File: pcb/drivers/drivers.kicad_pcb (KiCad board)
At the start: 2 copper layers, 51.4 x 53.3 mm, 20 parts, among them J1 Conn_01x04_Male, J2 Conn_01x04_Male, J3 Conn_01x04_Male, J4 Conn_01x04_Male, J5 Conn_01x04_Male, J6 Conn_01x02_Male, J7 Conn_01x12_Female, J8 Conn_01x12_Female, Q1 IRLML6402, Q2 IRLML6402, Q3 IRLML6402, Q4 IRLML6402, Q5 IRLML6402

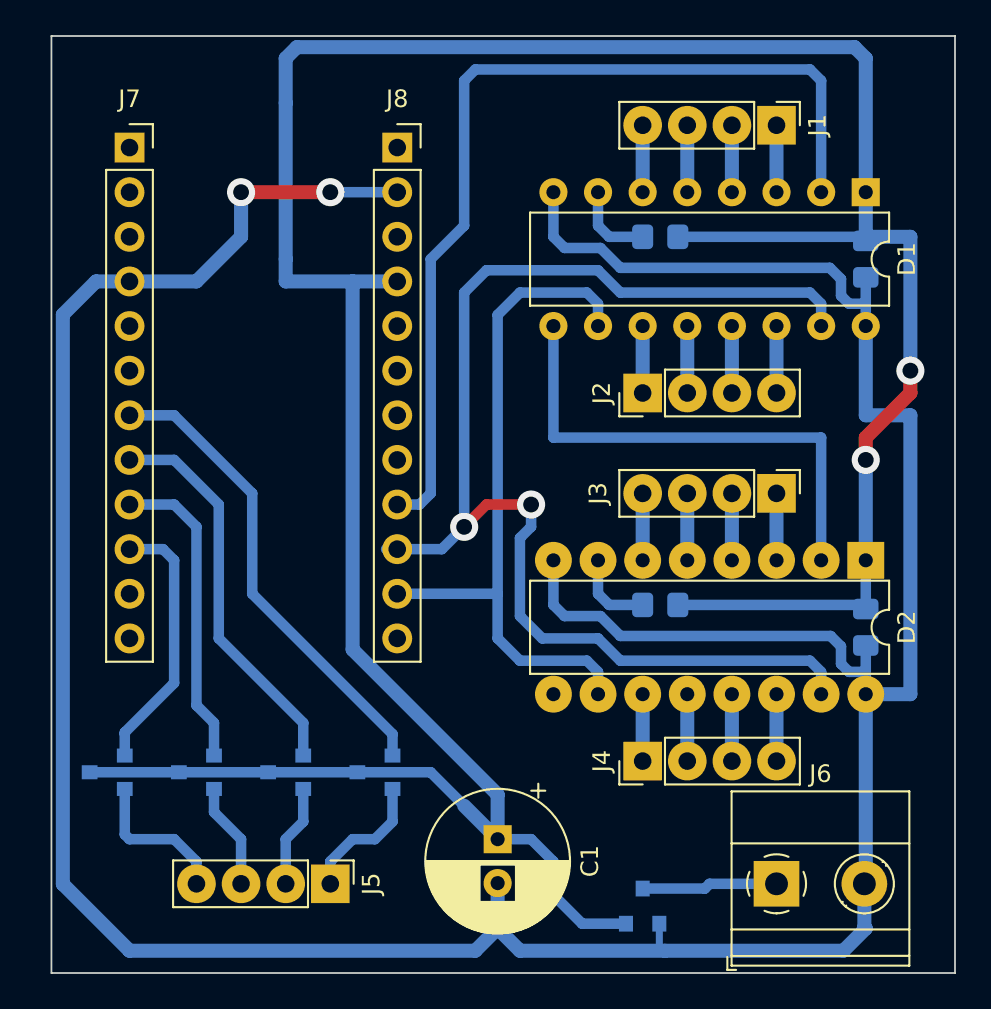
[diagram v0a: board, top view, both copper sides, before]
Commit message: Polishing
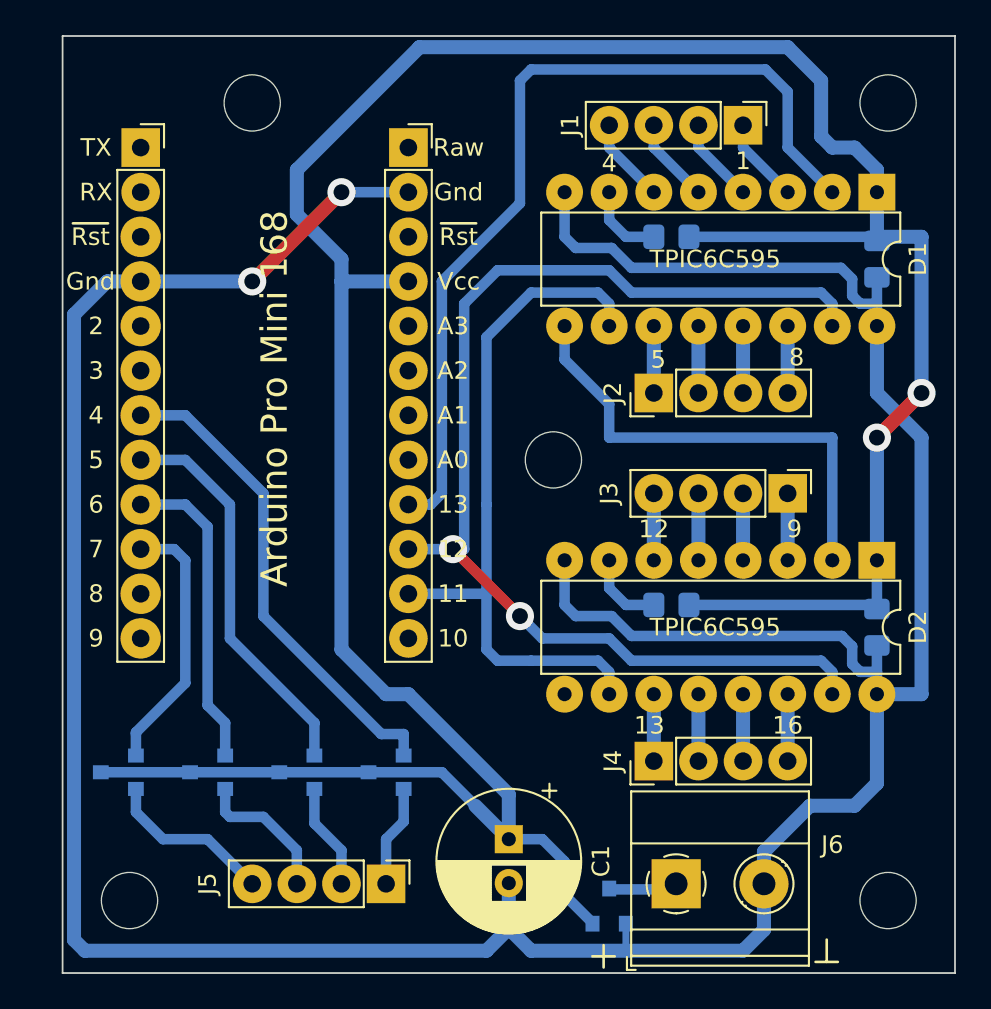
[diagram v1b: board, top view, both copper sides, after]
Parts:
- added H1: MountingHole, MountingHole:MountingHole_3.2mm_M3, F.Cu at (71.8, 31.8)
- added H2: MountingHole, MountingHole:MountingHole_3.2mm_M3, F.Cu at (88.9, 52.1)
- added H3: MountingHole, MountingHole:MountingHole_3.2mm_M3, F.Cu at (108.0, 31.8)
- added H4: MountingHole, MountingHole:MountingHole_3.2mm_M3, F.Cu at (64.8, 77.2)
- added H5: MountingHole, MountingHole:MountingHole_3.2mm_M3, F.Cu at (108.0, 77.2)
- moved J6 5.71 mm to (95.9, 76.2)
- moved J5 3.17 mm to (79.4, 76.2)
- moved J1 1.91 mm to (99.7, 33.0)
- moved Q5 1.91 mm to (92.1, 77.5)
- moved C1 0.64 mm to (86.4, 73.7)
- moved J3 0.64 mm to (102.2, 54.0)
- moved J7 0.64 mm to (65.4, 34.3)
- moved Q1 0.64 mm to (79.4, 69.8)
- moved Q2 0.64 mm to (74.3, 69.8)
- moved Q3 0.64 mm to (69.2, 69.8)
- moved Q4 0.64 mm to (64.1, 69.8)
- moved C2 0.63 mm to (107.3, 40.6)
- moved C3 0.63 mm to (107.3, 61.6)
- moved D1 0.63 mm to (107.3, 36.8)
- moved D2 0.63 mm to (107.3, 57.8)
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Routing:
- net VCC: track 179.1 -> 170.8 mm
- net /12: track 71.9 -> 66.7 mm
- net Net-(J6-Pad1): track 7.73 -> 3.54 mm
- net GND: track 198.4 -> 195.0 mm
- net /13: track 53.6 -> 50.3 mm
- net Net-(J5-Pad3): track 6.04 -> 8.21 mm
- net Net-(J5-Pad1): track 7.61 -> 5.81 mm
- net Net-(D1-Pad9): track 28.6 -> 27.1 mm
- net Net-(D1-Pad5): track 3.81 -> 4.86 mm
- net Net-(D1-Pad3): track 3.81 -> 4.86 mm
- net Net-(J5-Pad4): track 8.58 -> 9.63 mm
- net Net-(D1-Pad6): track 3.81 -> 4.86 mm
- net Net-(D1-Pad4): track 3.81 -> 4.86 mm
- net /11: track 39.7 -> 40.6 mm
- net /4: track 27.1 -> 27.8 mm
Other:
- board size 51.4 x 53.3 mm -> 50.8 x 53.3 mm
- board text added: "1"
- board text added: "10"
- board text added: "11"
- board text added: "12"
- board text added: "13"
- board text added: "16"
- board text added: "2"
- board text added: "3"
- board text added: "4"
- board text added: "5"
- board text added: "6"
- board text added: "7"
- board text added: "8"
- board text added: "9"
- board text added: "A0"
- board text added: "A1"
- board text added: "A2"
- board text added: "A3"
- board text added: "Arduino Pro Mini 168"
- board text added: "Gnd"
- board text added: "RX"
- board text added: "Raw"
- board text added: "TPIC6C595"
- board text added: "TX"
- board text added: "Vcc"
- board text added: "~Rst"
